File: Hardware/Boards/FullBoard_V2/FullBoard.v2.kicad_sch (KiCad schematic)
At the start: 20 parts, among them J2 Conn_01x03_Pin, K1 Relay_SPDT, K2 Relay_SPDT, K3 Relay_SPDT, K4 Relay_SPDT, U2 DS18B20-air, U2 DS18B20-water, U4 TEMT6000, U5 GY-8511 UV sensor, U6 Turbidity sensor, U7 Water Level

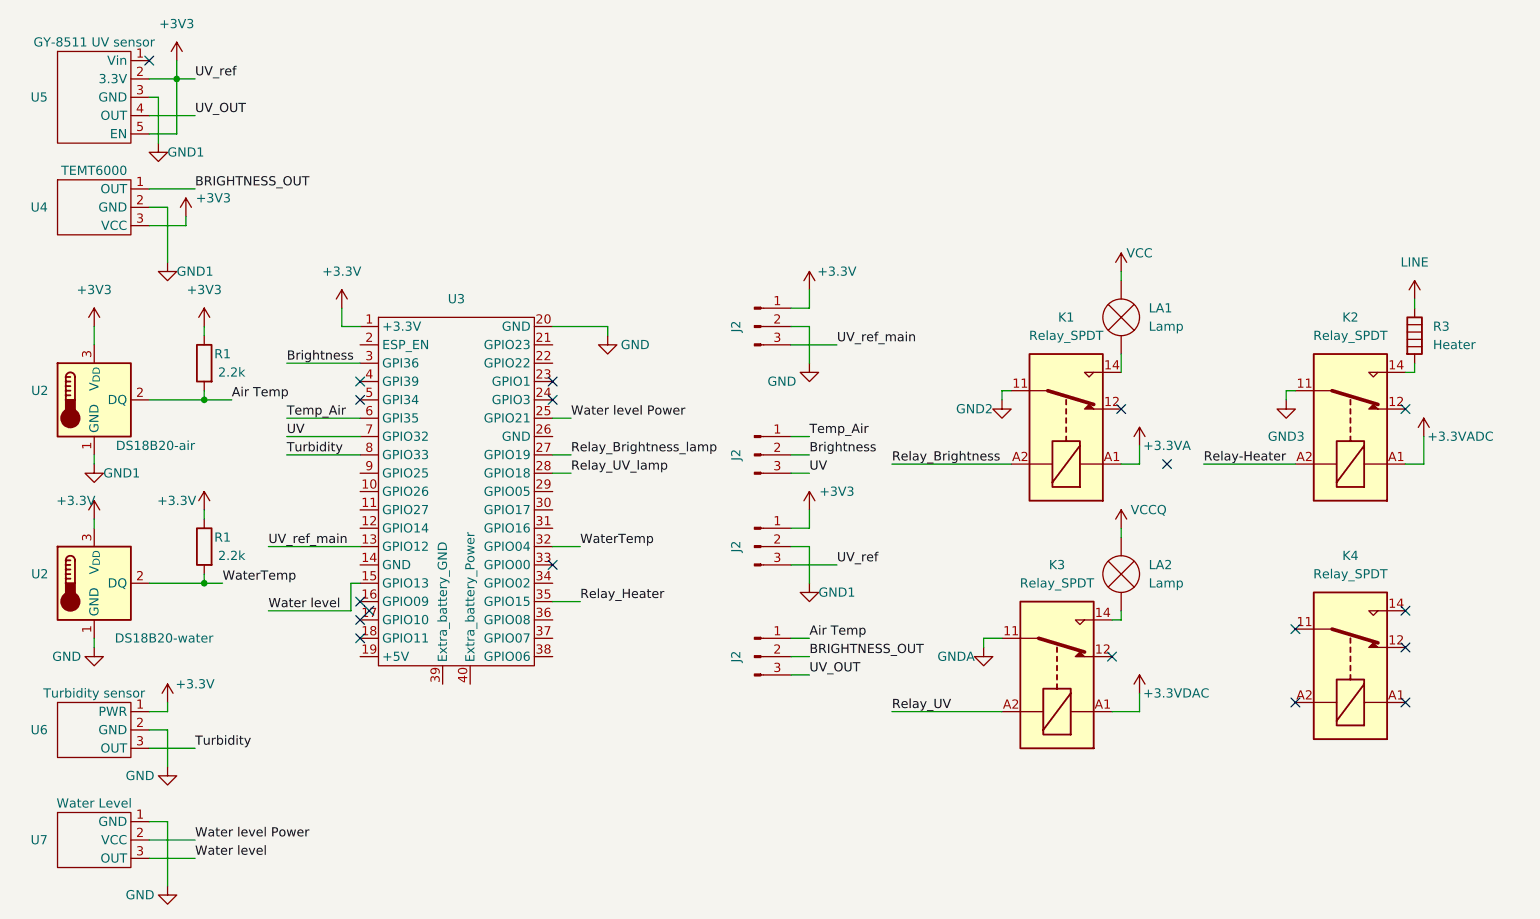
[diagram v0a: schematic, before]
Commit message: Almost completed scheme
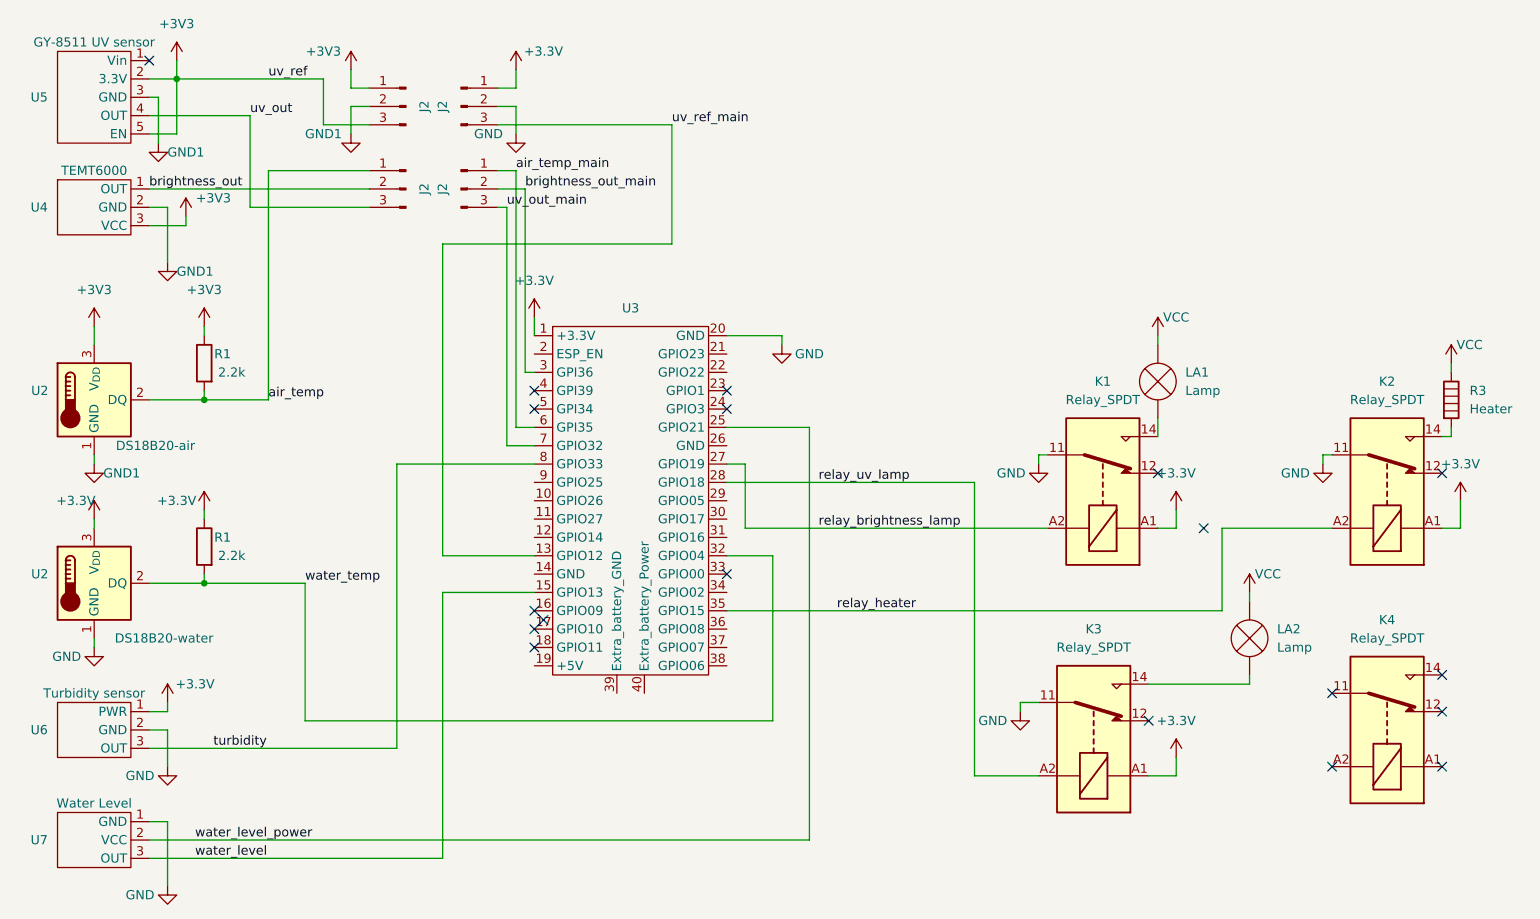
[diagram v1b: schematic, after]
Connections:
- net +3.3VA is gone; now on net +3.3V: K1.A1
- net +3.3VADC is gone; now on net +3.3V: K2.A1
- net +3.3VDAC is gone; now on net +3.3V: K3.A1
- net GND2 is gone; now on net GND: K1.11
- net GND3 is gone; now on net GND: K2.11
- net GNDA is gone; now on net GND: K3.11
- net LINE is gone; now on net VCC: R3.1
- net Relay_Brightness_lamp is gone; now on net relay_brightness_lamp: U3.27 (GPIO19)
- net Relay_Heater is gone; now on net relay_heater: U3.35 (GPIO15)
- net Relay_UV_lamp is gone; now on net relay_uv_lamp: U3.28 (GPIO18)
- net VCCQ is gone; now on net VCC: LA2.2 (+)
- net Air Temp renamed air_temp
- net BRIGHTNESS_OUT renamed brightness_out
- net Brightness renamed brightness_out_main
- net Relay-Heater renamed relay_heater
- net Relay_Brightness renamed relay_brightness_lamp
- net Relay_UV renamed relay_uv_lamp
- net Temp_Air renamed air_temp_main
- net Turbidity renamed turbidity
- net UV renamed uv_out_main
- net UV_OUT renamed uv_out
- net UV_ref_main renamed uv_ref_main
- net Water level renamed water_level
- net Water level Power renamed water_level_power
- net WaterTemp renamed water_temp
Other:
- moved on the sheet: J2, K1, K2, K3, K4, LA1, LA2, R3, U3
